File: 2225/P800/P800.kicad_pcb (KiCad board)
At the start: 2 copper layers, 115 x 82.5 mm, 29 parts, among them J1 Screw_Terminal_01x05, J2 Conn_Coaxial, J3 Conn_Coaxial, J4 Conn_Coaxial, J5 Conn_Coaxial

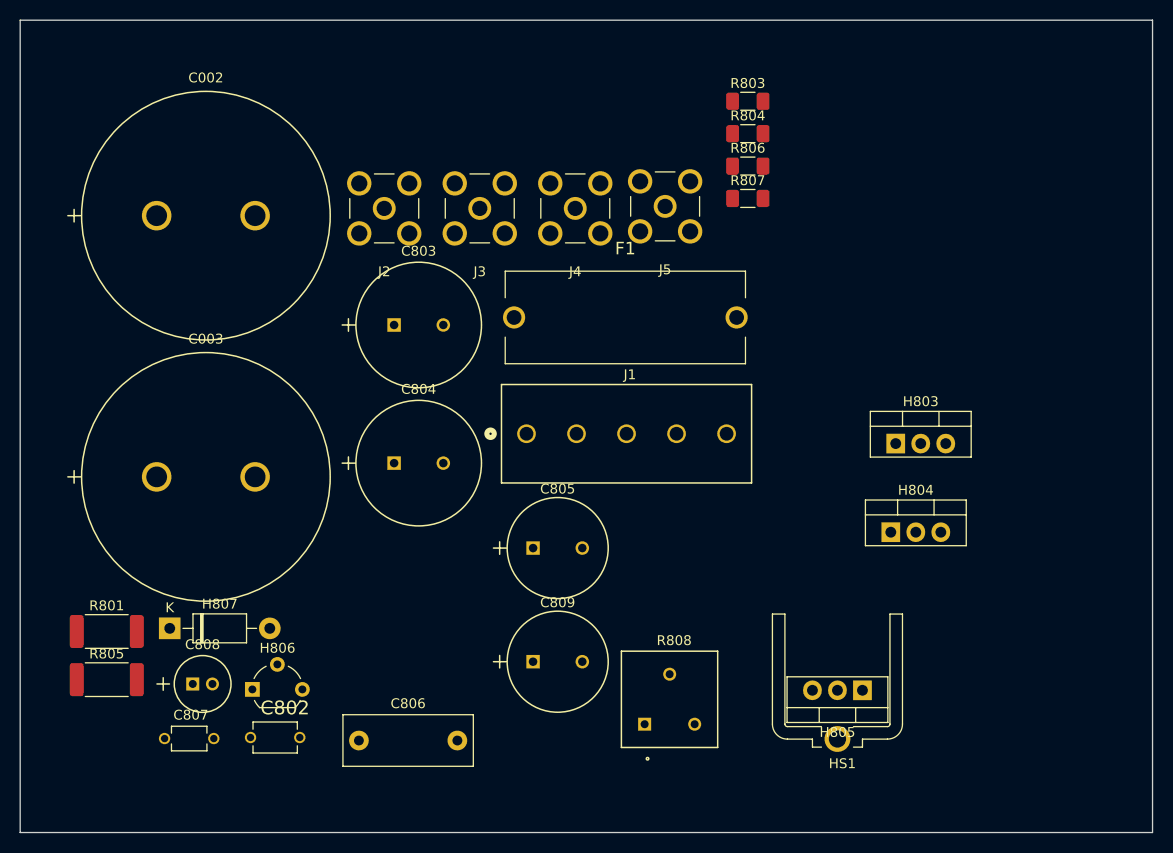
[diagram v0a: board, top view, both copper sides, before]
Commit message: Completed initial P800 board layout.
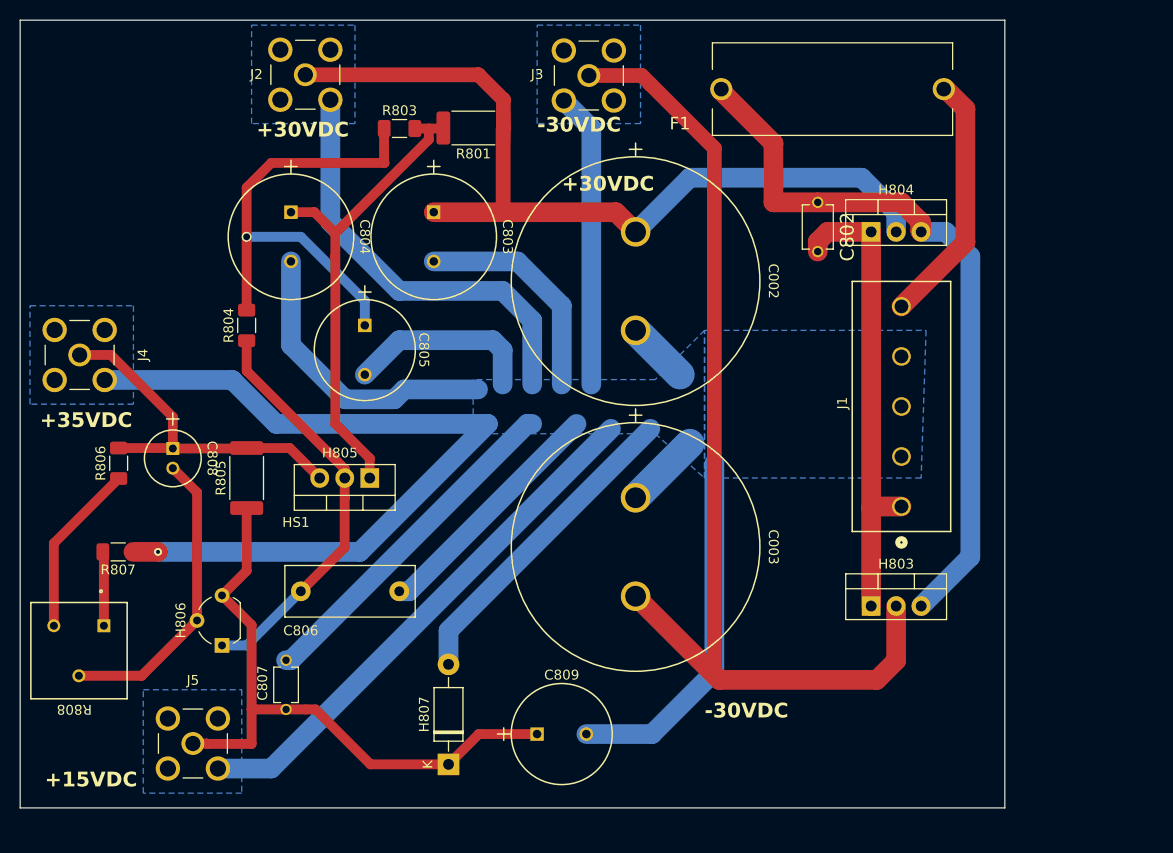
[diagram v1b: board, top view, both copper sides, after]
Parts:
- HS1: value Heatsink_Pad -> Heatsink; footprint P800_footprint_library:heatsink_577202B04000G -> P800_footprint_library:heatsink_577202B00000G
- moved C802 75.7 mm to (104.5, 37.5), turned to -90 degrees
- moved R807 73.3 mm to (33.5, 70.5), turned to 180 degrees
- moved J5 72.6 mm to (41.0, 90.0), turned to 0 degrees
- moved R806 70.7 mm to (33.5, 61.5), turned to 90 degrees
- moved R801 63.3 mm to (69.5, 27.4), turned to 180 degrees
- moved R808 55.8 mm to (32.0, 78.0), turned to 180 degrees
- moved HS1 54.5 mm to (56.5, 67.8)
- moved R804 54.5 mm to (46.5, 47.5), turned to 90 degrees
- moved H805 54.5 mm to (59.0, 63.0)
- moved J4 52.5 mm to (29.5, 50.5), turned to -90 degrees
- moved C003 48.7 mm to (86.0, 65.0), turned to -90 degrees
- moved C002 48.7 mm to (86.0, 38.0), turned to -90 degrees
- moved J1 38.8 mm to (113.0, 65.9), turned to 90 degrees
- moved R803 35.5 mm to (62.0, 27.5)
- moved H807 31.5 mm to (67.0, 92.1), turned to 90 degrees
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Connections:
- C802 pad 1: Net-(C802-Pad1) -> /+24VAC
- F1 pad 1: /+24VAC -> Net-(J1-Pin_5)
- F1 pad 2: Net-(C802-Pad1) -> /+24VAC
- H803 pad 3: Net-(C802-Pad1) -> /+24VAC
- H804 pad 3: Net-(C802-Pad1) -> /+24VAC
- J1 pad 5: /+24VAC -> Net-(J1-Pin_5)
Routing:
- net GND: track 0.00 -> 425.7 mm, vias 0 -> 1
- net /-30VDC_out: track 0.00 -> 105.6 mm
- net /+30VDC_out: track 0.00 -> 86.1 mm
- net /+24VAC: track 0.00 -> 76.1 mm
- net /15VDC_out: track 0.00 -> 64.8 mm
- net Net-(H805-C): track 0.00 -> 49.2 mm
- net Net-(C805-Pad1): track 0.00 -> 48.2 mm, vias 0 -> 1
- net /-24VAC: track 0.00 -> 48.1 mm
- net Net-(H805-B): track 0.00 -> 41.7 mm
- net /35VDC_out: track 0.00 -> 36.9 mm
- net Net-(H806-B): track 0.00 -> 30.8 mm
- net Net-(J1-Pin_5): track 0.00 -> 25.8 mm
- net Net-(R806-Pad1): track 0.00 -> 17.7 mm
- net Net-(R807-Pad2): track 0.00 -> 7.54 mm
- added copper zone on B.Cu, net GND
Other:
- board size 115 x 82.5 mm -> 100 x 80 mm
- board text added: "+15VDC"
- board text added: "+30VDC"
- board text added: "+35VDC"
- board text added: "-30VDC"
